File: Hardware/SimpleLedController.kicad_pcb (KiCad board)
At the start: 4 copper layers, 90 x 50 mm, 180 parts, among them J1 Jack-DC, J12 Screw_Terminal_01x02, J13 Screw_Terminal_01x02, J14 Screw_Terminal_01x02, J2 Molex KK2.54 4p male, J3 Connector, USB-TYPE-C-16P, J4 Servo1, J5 Screw_Terminal_01x03, J6 Conn_01x06, Q10 AO3400, Q3 AO3400, Q4 MMBT3906, Q5 MMBT3904, Q6 MMBT3904, Q7 MMBT3904, Q9 MMBT3904, SW1 RESET, SW3 RESET, SW4 RESET, U1 LM74700, U10 INA219AxDCN, U18 CH340G, U19 SL2.1A, U2 LM74700, U22 ESP32-S3-WROOM-1, U24 DRV8870DDA, U25 SN74LVC1G00DBV, U26 SN74LVC1G00DBV, U27 DRV8870DDA, U28 SN74LVC1G00DBV, U29 SN74LVC1G00DBV, U3 IP2721, U30 DRV8870DDA, U31 SN74LVC1G00DBV, U32 SN74LVC1G00DBV, U4 IP4234CZ6, U5 TPS56339, U6 TPS56339, U7 INA219AxDCN, U8 SN74LVC1G00DBV, U9 INA219AxDCN, Y1 12MHz C7424717, Y2 12MHz C7424717

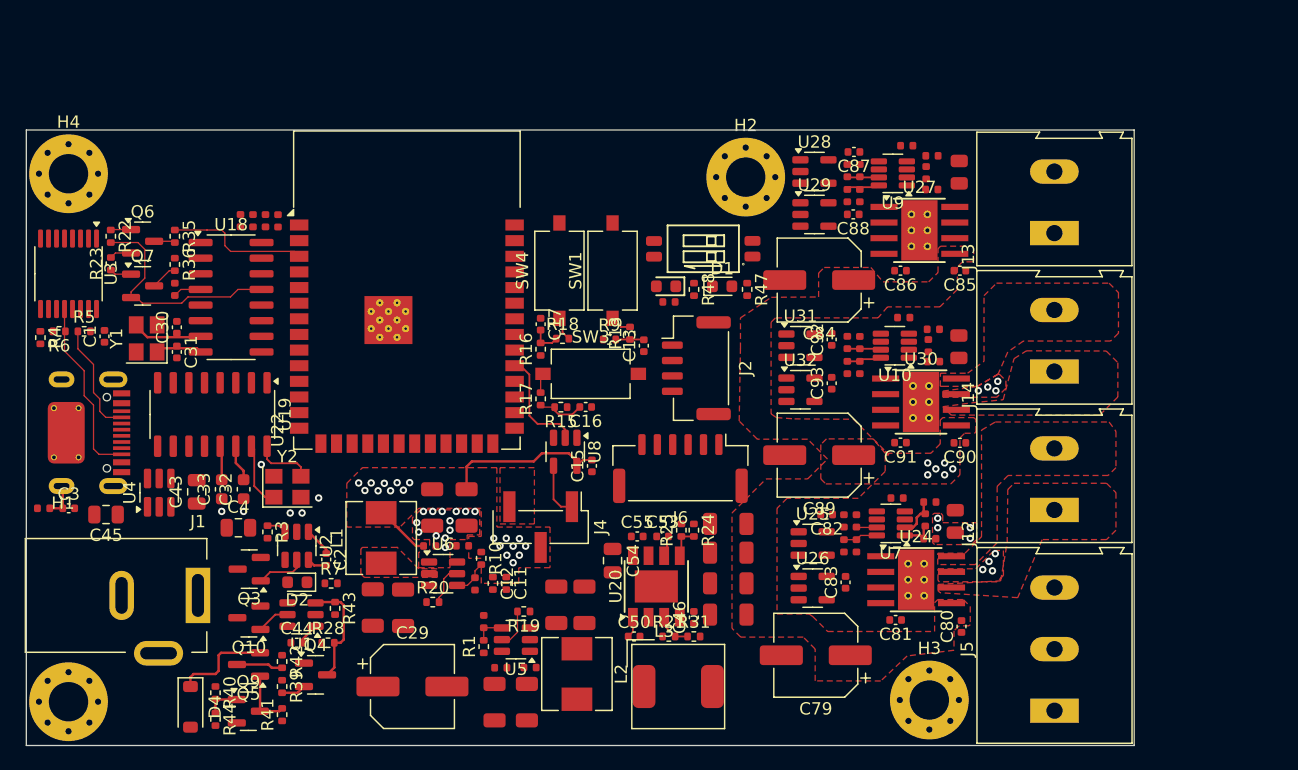
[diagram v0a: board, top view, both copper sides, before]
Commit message: Finish PCB
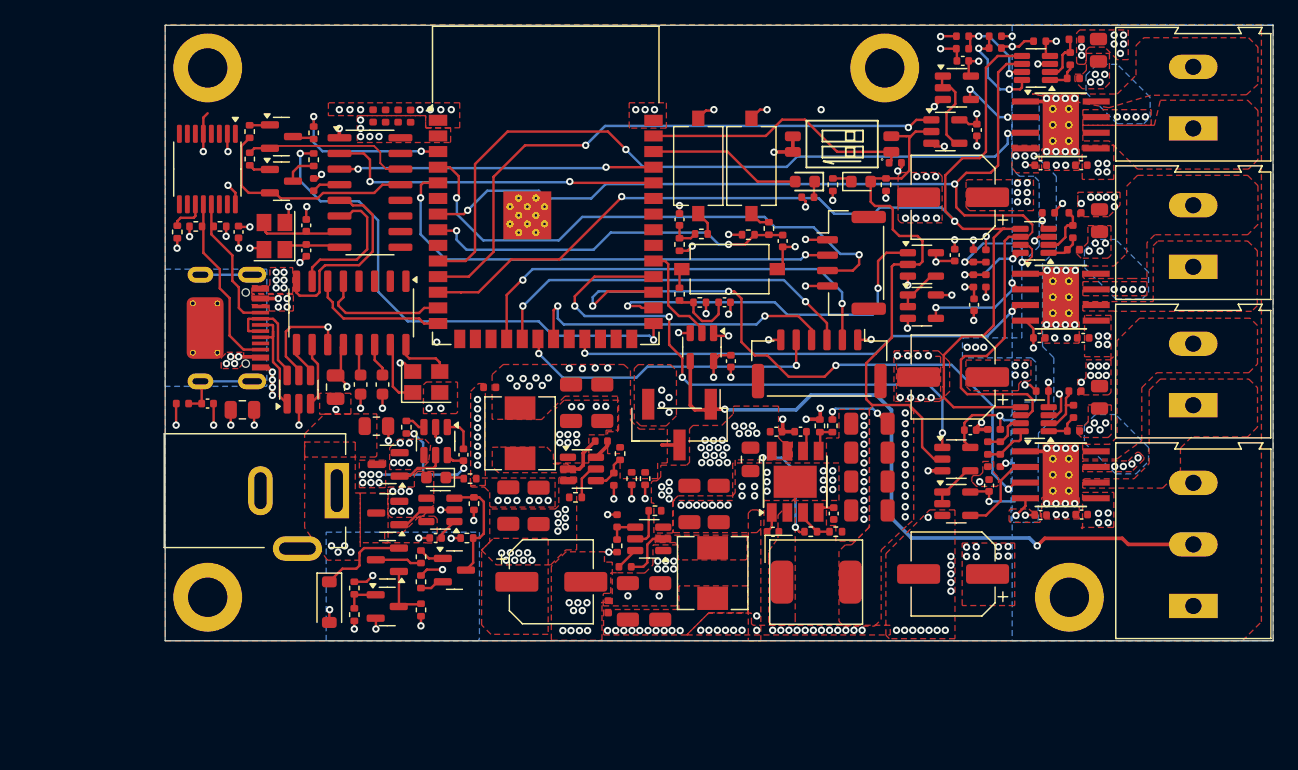
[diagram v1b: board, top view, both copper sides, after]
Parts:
- removed the G*** at (125.2, 94.0)
- removed the G*** at (132.8, 95.8)
- added G***: LOGO, Logo:SilkLogo2, B.Cu at (149.0, 104.0)
- added G***: LOGO, Logo:SilkLogo1, B.Cu at (143.0, 82.0)
- added R12: 10kΩ, PCM_JLCPCB:R_0402, F.Cu at (158.9, 73.0)
- added REF**: My_github, Symbol:My_github, B.Cu at (139.0, 94.6)
- added REF**: WEEE-Logo_5.6x8mm_SilkScreen, Symbol:WEEE-Logo_5.6x8mm_SilkScreen, B.Cu at (121.0, 104.0)
- added REF**: ESD-Logo_8.9x8mm_SilkScreen, Symbol:ESD-Logo_8.9x8mm_SilkScreen, B.Cu at (129.0, 104.0)
- H1, H2, H3, H4: footprint MountingHole:MountingHole_3.2mm_M3_Pad_Via -> MountingHole:MountingHole_3.2mm_M3_DIN965_Pad
- moved R55 17.0 mm to (167.0, 62.7), turned to 180 degrees
- moved R32 17.0 mm to (167.0, 63.7), turned to 0 degrees
- moved U29 15.5 mm to (163.9, 66.9)
- moved R50 15.5 mm to (175.4, 92.1)
- moved R52 15.3 mm to (175.4, 77.7)
- moved C88 15.3 mm to (164.3, 64.7), turned to 0 degrees
- moved J2 15.2 mm to (155.3, 81.2)
- moved R51 15.0 mm to (175.4, 63.9)
- moved R46 15.0 mm to (173.5, 63.0)
- moved C28 15.0 mm to (173.3, 78.6)
- moved C27 14.9 mm to (173.1, 64.6)
- moved C26 14.9 mm to (173.3, 93.2)
- moved R49 14.9 mm to (173.5, 77.1)
- moved R45 14.8 mm to (173.5, 91.6)
- moved C23 14.7 mm to (170.8, 91.6)
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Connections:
- H2 pad 1: GND -> unconnected-(H2-Pad1)
- H3 pad 1: GND -> unconnected-(H3-Pad1)
- H4 pad 1: GND -> unconnected-(H4-Pad1)
- S1 pad 1: /MCU/POWER SECTION/DRV1/~{SAFE OPERATION} -> /MCU/5V WS2812 and Servo/Other.USER_SW
- U22 pad 39: /MCU/5V WS2812 and Servo/Other.BUZZER -> /MCU/5V WS2812 and Servo/Other.USER_SW
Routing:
- net /MCU/ESP32S3/I2C1.SCL: track 0.00 -> 93.8 mm, vias 0 -> 2
- net /MCU/ESP32S3/I2C1.SDA: track 0.00 -> 92.0 mm, vias 0 -> 2
- net GND: track 0.00 -> 85.4 mm, vias 19 -> 262
- net /MCU/ESP32S3/Hbridge1.IN1: track 0.00 -> 59.1 mm, vias 0 -> 2
- net /MCU/ESP32S3/Hbridge3.IN1: track 0.00 -> 54.5 mm, vias 0 -> 4
- net /MCU/5V WS2812 and Servo/5V Data/PWM: track 4.47 -> 56.1 mm, vias 0 -> 2
- net +3V3: track 0.09 -> 49.8 mm, vias 0 -> 48
- net /MCU/ESP32S3/Hbridge1.IN2: track 0.00 -> 49.0 mm, vias 0 -> 2
- net /MCU/ESP32S3/Hbridge3.IN2: track 0.00 -> 47.1 mm, vias 0 -> 4
- net /MCU/ESP32S3/I2C2.SDA: track 0.00 -> 44.3 mm, vias 0 -> 2
- net /MCU/POWER SECTION/DRV1/~{SAFE OPERATION}: track 0.00 -> 43.9 mm
- net /MCU/CH340 prog/UART_PROG.BOOT: track 0.00 -> 42.1 mm, vias 0 -> 2
- net /MCU/ESP32S3/I2C2.SCL: track 0.00 -> 39.6 mm, vias 0 -> 2
- net /MCU/ESP32S3/Hbridge2.IN1: track 0.00 -> 38.6 mm, vias 0 -> 2
- net /MCU/ESP32S3/VSPI.CS: track 0.00 -> 36.3 mm, vias 0 -> 2
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- added copper zone on In2.Cu, net +12V
- added copper zone on B.Cu, net +3V3
- added copper zone on F.Cu, net +3V3
- added copper zone on In2.Cu, net +3V3
- added copper zone on In2.Cu, net +5V
- added copper zone on B.Cu, net /USB_PD/UVP-OVP/Vin
- added copper zone on F.Cu, net /USB_PD/UVP-OVP/Vin
- added copper zone on In2.Cu, net /USB_PD/UVP-OVP/Vin
- added copper zone on F.Cu, net /USB_PD/VBUS
- added copper zone on In2.Cu, net /USB_PD/VBUS
- added copper zone on B.Cu, net GND
- added copper zone on F.Cu, net Net-(J13-Pin_1)
- added copper zone on F.Cu, net Net-(J13-Pin_2)
- added copper zone on B.Cu, net Net-(J3-SHIELD)
- added copper zone on F.Cu, net Net-(Q3-S)
- added copper zone on In2.Cu, net Net-(Q3-S)
- added copper zone on F.Cu, net Net-(U20-Lx)
- added copper zone on B.Cu, net Net-(U24-ISEN)
- added copper zone on B.Cu, net Net-(U27-ISEN)
- added copper zone on F.Cu, net Net-(U27-ISEN)
- added copper zone on B.Cu, net Net-(U30-ISEN)
- added copper zone on F.Cu, net Net-(U5-SW)
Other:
- board text added: "10-02-2025"
- board text added: "9mm Label"
- board text added: "BRD REV:A"
- board text added: "BY ARTEM H."
- board text added: "DESIGNED IN POLAND"
- board text added: "JLCJLCJLCJLC"
- board text added: "MADE IN CHINA BY JLCPCB"
